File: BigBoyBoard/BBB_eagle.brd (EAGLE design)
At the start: 94 x 87.1 mm, 36 parts, among them Y2 ECS-80-S-4X

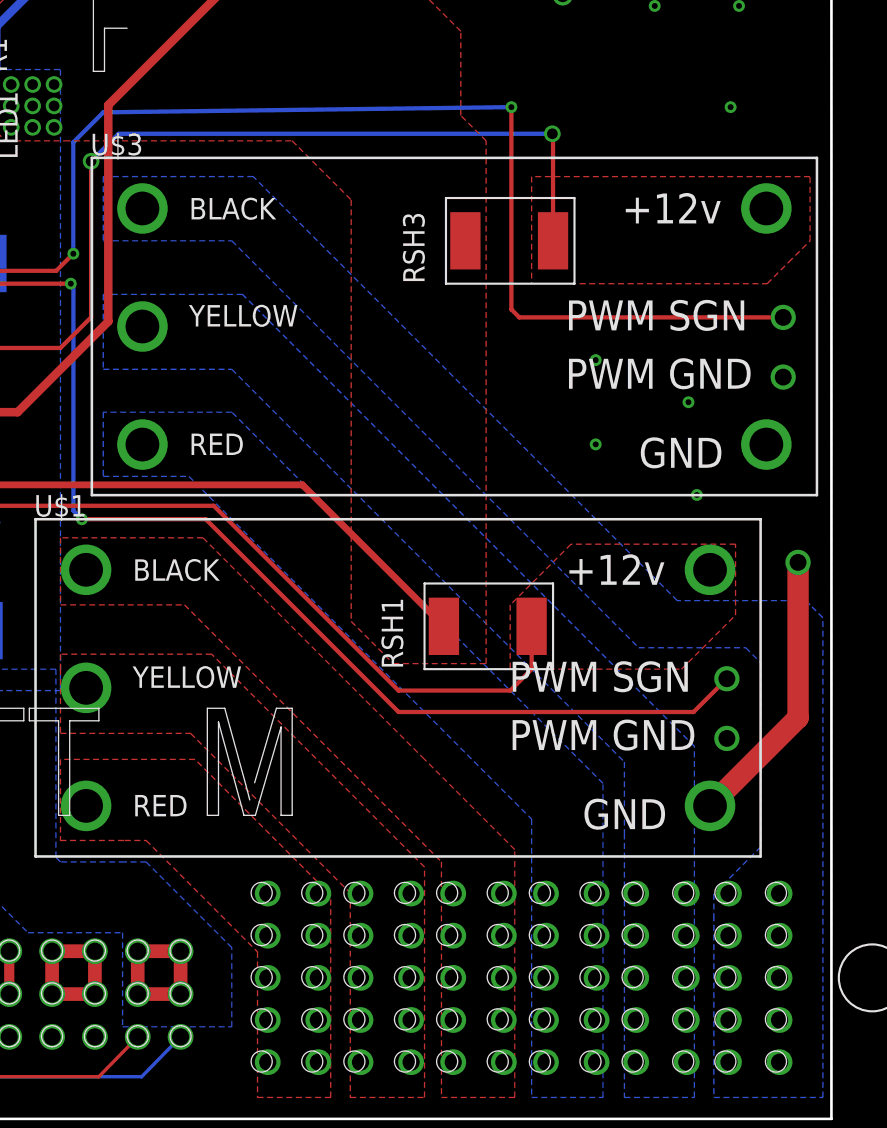
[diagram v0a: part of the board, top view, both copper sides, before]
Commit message: Update BigBoyBoard/BBB_eagle.brd
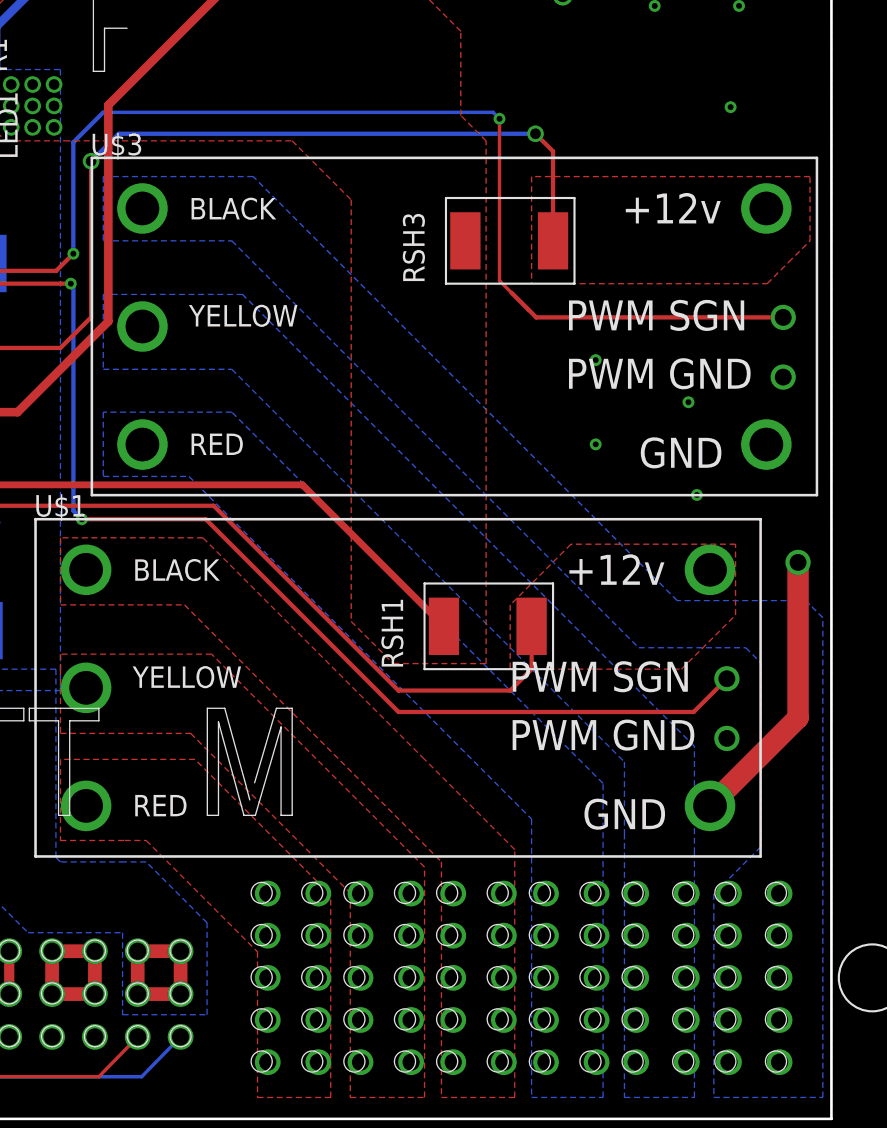
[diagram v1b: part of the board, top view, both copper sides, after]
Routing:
- net VCC3: track 74.1 -> 73.5 mm
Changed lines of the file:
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@@
 <wire x1="52.842" y1="7.403" x2="55.382" y2="7.403" width="0.8128" layer="1"/>
 <polygon width="0.508" layer="16" thermals="no">
-<vertex x="58.42" y="5.461"/>
-<vertex x="58.42" y="10.16"/>
+<vertex x="56.951" y="6.176"/>
+<vertex x="56.951" y="11.629"/>
 <vertex x="53.34" y="15.24"/>
 <vertex x="52.07" y="15.24"/>
@@
 <vertex x="46.338" y="11.04"/>
 <vertex x="51.943" y="11.04"/>
-<vertex x="51.943" y="5.461"/>
+<vertex x="51.943" y="6.176"/>
 </polygon>
 <contactref element="U$6" pad="R6-6"/>
@@
 <wire x1="32.92" y1="57.25" x2="32.92" y2="58.24" width="0.254" layer="1"/>
 <wire x1="39.878" y1="50.292" x2="32.92" y2="57.25" width="0.254" layer="1"/>
-<wire x1="50.8" y1="59.69" x2="75" y2="60" width="0.254" layer="16"/>
-<via x="75" y="60" extent="1-16" drill="0.35"/>
-<wire x1="75" y1="48" x2="75" y2="60" width="0.254" layer="1"/>
-<wire x1="91.12" y1="47.53" x2="75.47" y2="47.53" width="0.254" layer="1"/>
-<wire x1="75.47" y1="47.53" x2="75" y2="48" width="0.254" layer="1"/>
+<wire x1="91.12" y1="47.53" x2="76.47" y2="47.53" width="0.254" layer="1"/>
+<wire x1="76.47" y1="47.53" x2="76" y2="48" width="0.254" layer="1"/>
+<wire x1="76" y1="48" x2="75" y2="49" width="0.254" layer="1"/>
+<wire x1="50.8" y1="59.69" x2="73.914" y2="59.69" width="0.2032" layer="16"/>
+<via x="74.295" y="59.309" extent="1-16" drill="0.35"/>
+<wire x1="74.295" y1="59.309" x2="74.295" y2="49.705" width="0.2032" layer="1"/>
+<wire x1="74.295" y1="49.705" x2="76" y2="48" width="0.2032" layer="1"/>
+<wire x1="73.914" y1="59.69" x2="74.295" y2="59.309" width="0.2032" layer="16"/>
 </signal>
 <signal name="TIM3_CH3">
@@
 <via x="50.076" y="56.792" extent="1-16" drill="0.635"/>
 <wire x1="50.076" y1="56.792" x2="51.704" y2="58.42" width="0.254" layer="16"/>
-<wire x1="51.704" y1="58.42" x2="77.43" y2="58.42" width="0.254" layer="16"/>
-<via x="77.43" y="58.42" extent="1-16" drill="0.635"/>
-<wire x1="77.43" y1="58.42" x2="77.47" y2="58.38" width="0.254" layer="1"/>
-<wire x1="77.47" y1="58.38" x2="77.47" y2="52.07" width="0.254" layer="1"/>
+<wire x1="51.704" y1="58.42" x2="76.43" y2="58.42" width="0.254" layer="16"/>
+<via x="76.43" y="58.42" extent="1-16" drill="0.635"/>
+<wire x1="76.43" y1="58.42" x2="77.47" y2="57.38" width="0.254" layer="1"/>
+<wire x1="77.47" y1="57.38" x2="77.47" y2="52.07" width="0.254" layer="1"/>
 </signal>
 <signal name="VCC2">
